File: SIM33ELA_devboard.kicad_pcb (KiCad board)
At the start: 4 copper layers, 82.3 x 24.9 mm, 26 parts, among them J2 Conn_01x13_Pin, U2 SIM33ELA

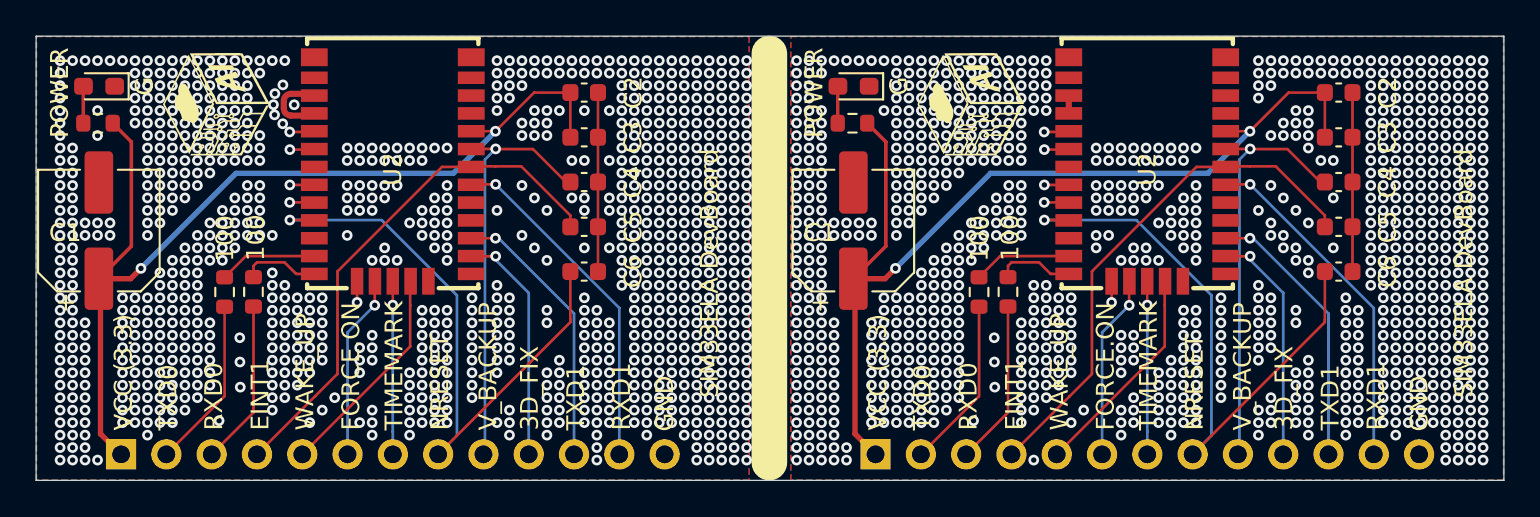
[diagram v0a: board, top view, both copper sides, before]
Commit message: cambios finales
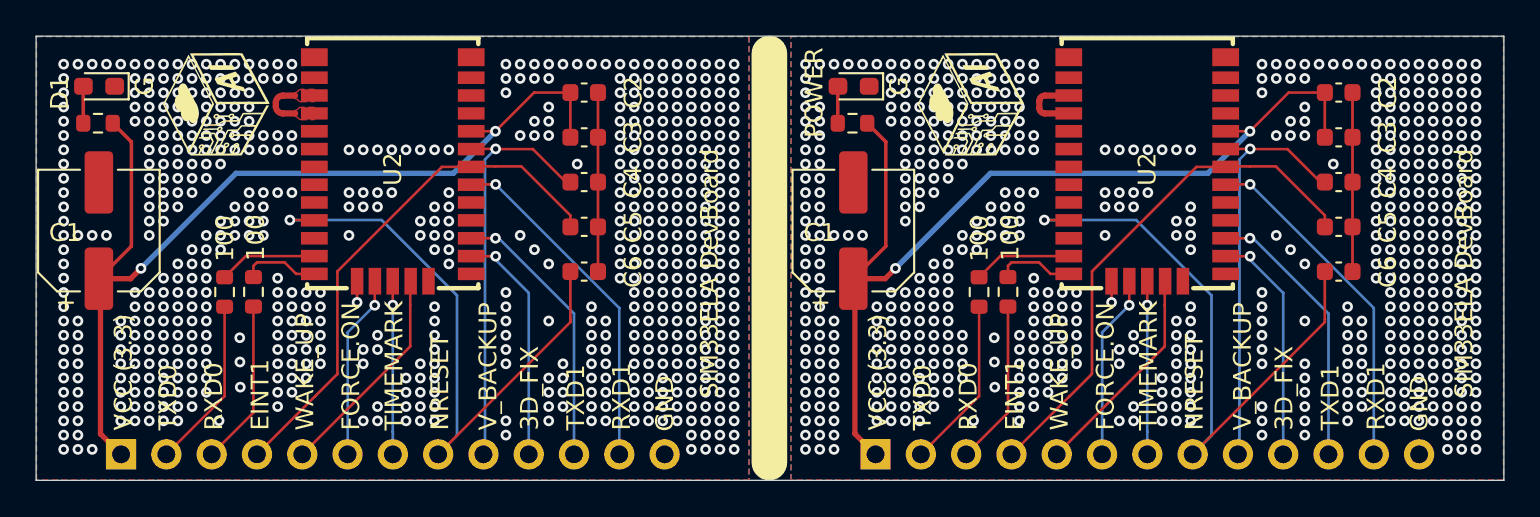
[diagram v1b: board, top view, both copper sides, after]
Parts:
- R3: value 2.7k -> 4.7k
- renumbered POWER to D1
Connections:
- U2 pad 16: Net-(U2-ANT) -> /RF_SIGNAL1
- U2 pad 17: Net-(U2-ANT) -> /RF_SIGNAL1
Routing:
- net GND: track 33.3 -> 22.5 mm, vias 1886 -> 1201
- net /RF_SIGNAL1: track 0.00 -> 4.14 mm
- net Net-(U2-ANT): track 6.56 -> 4.02 mm
- added copper zone on F.Cu, net /RF_SIGNAL1

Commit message: diseño final
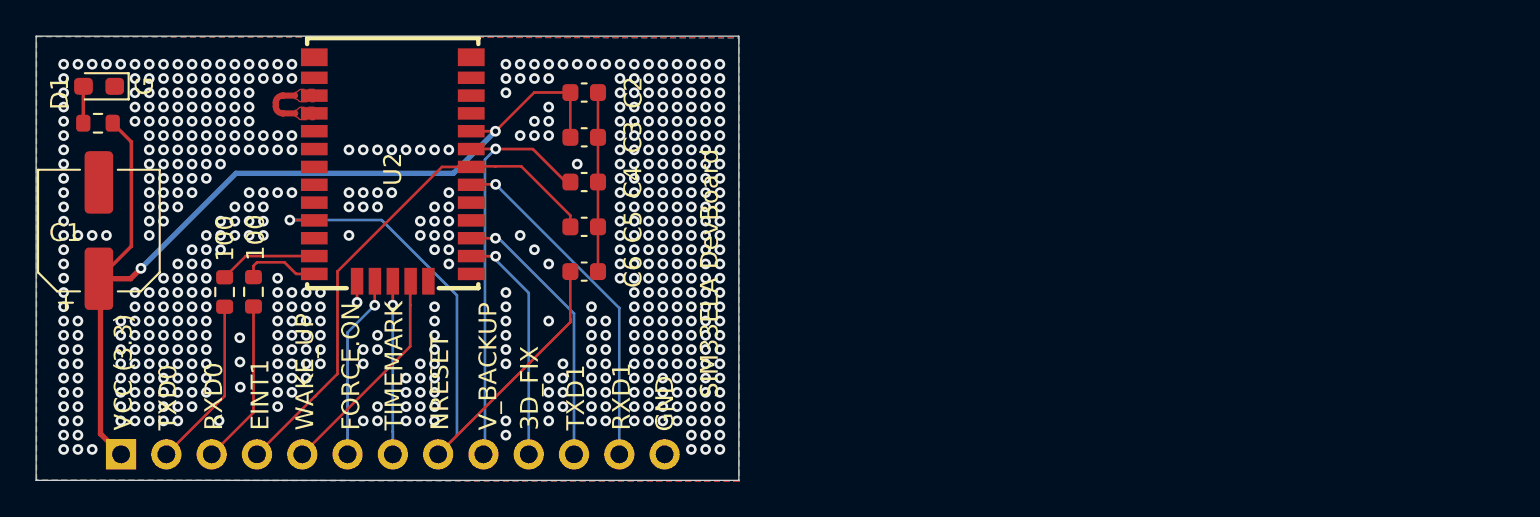
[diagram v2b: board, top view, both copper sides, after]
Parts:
- removed the C1 at (170.6, 91.8)
- removed the C2 at (197.8, 84.0)
- removed the C3 at (197.8, 86.5)
- removed the C4 at (197.8, 89.0)
- removed the C5 at (197.8, 91.5)
- removed the C6 at (197.8, 94.1)
- removed G*** (x2): LOGO, Images:LOGOv3.4
- removed the J2 at (171.8, 104.3)
- removed POWER: LED_Small, LED_SMD:LED_0603_1608Metric_Pad1.05x0.95mm_HandSolder
- removed the R1 at (179.3, 95.2)
- removed the R2 at (177.7, 95.2)
- removed the R3 at (170.6, 85.7)
- removed the U2 at (187.1, 88.3)
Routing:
- net /VCC: track 109.7 -> 54.9 mm, vias 4 -> 2
- net /NRESET: track 70.3 -> 35.2 mm, vias 2 -> 1
- net /EINT1: track 58.8 -> 29.4 mm
- net /V_BAKCUP: track 47.5 -> 23.7 mm, vias 2 -> 1
- net /RXD1: track 38.7 -> 19.4 mm, vias 2 -> 1
- net /TXD1: track 30.8 -> 15.4 mm, vias 2 -> 1
- net /3D-FIX: track 26.5 -> 13.2 mm, vias 2 -> 1
- net /WAKE_UP: track 24.5 -> 12.2 mm
- net GND: track 22.5 -> 11.2 mm, vias 1201 -> 581
- net /FORCE_ON: track 20.7 -> 10.4 mm, vias 2 -> 1
- net /TIMEMARK: track 19.5 -> 9.73 mm, vias 2 -> 1
- net /TXD0: track 19.3 -> 9.63 mm
- net /RXD0: track 18.5 -> 9.26 mm
- net Net-(U2-TXD0): track 11.0 -> 5.52 mm
- net Net-(U2-RXD0): track 8.78 -> 4.39 mm
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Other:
- board size 82.3 x 24.9 mm -> 39.4 x 24.9 mm
- board text removed: "recto"

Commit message: aaa
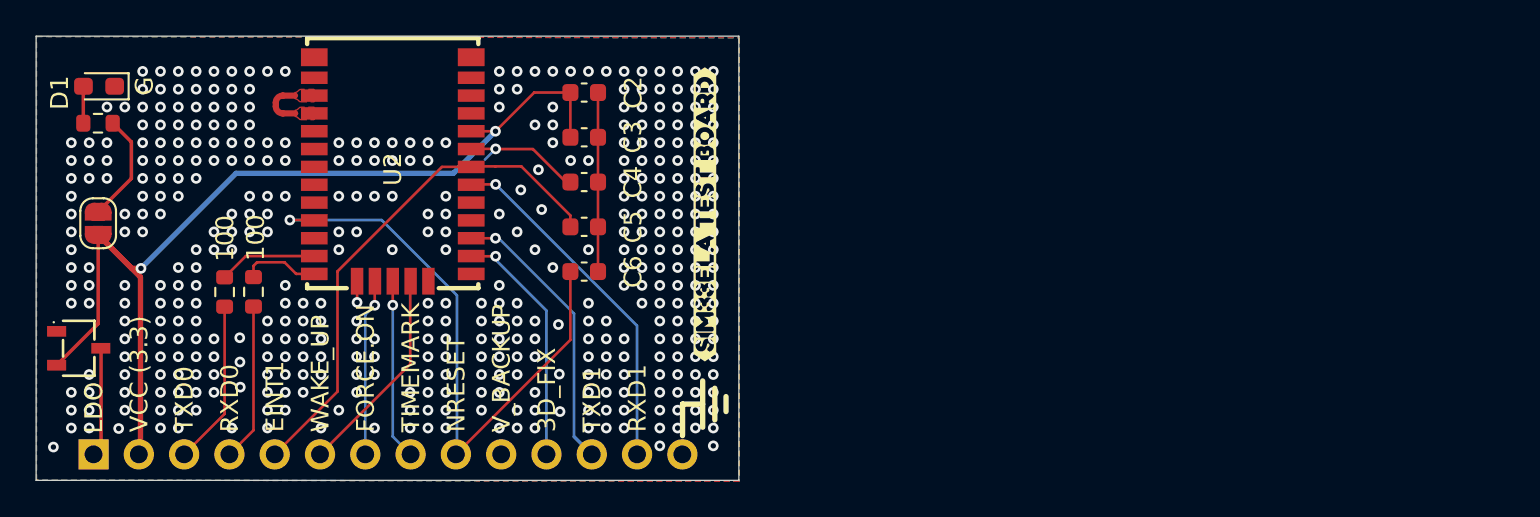
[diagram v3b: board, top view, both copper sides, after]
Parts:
- removed C1: 470uF, Capacitor_SMD:CP_Elec_6.3x7.7
- removed J2: Conn_01x13_Pin, Connector_PinHeader_2.54mm:PinHeader_1x13_P2.54mm_Vertical
- added J1: Conn_01x14_Pin, Connector_PinHeader_2.54mm:PinHeader_1x14_P2.54mm_Vertical, B.Cu at (128.0, 104.3)
- added JP1: SolderJumper_2_Open, Jumper:SolderJumper-2_P1.3mm_Open_RoundedPad1.0x1.5mm, F.Cu at (128.2, 91.3)
- added U1: XC6206P332MR, EasyEDA:SOT-23-3_L2.9-W1.6-P1.90-LS2.8-BR, F.Cu at (127.2, 98.4)
- added kibuzzard-6A1C62F4: G***, kibuzzard-6A1C62F4, F.Cu at (162.3, 90.8)
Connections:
- R3 pad 2: /VCC -> Net-(JP1-A)
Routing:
- net /V_BAKCUP: track 23.7 -> 7.17 mm
- net Net-(JP1-A): track 0.00 -> 6.16 mm
- net /LDO: track 0.00 -> 6.13 mm
- net /VCC: track 54.9 -> 56.9 mm
- net /NRESET: track 35.2 -> 34.3 mm
- net GND: vias 581 -> 420
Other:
- board text added: "LDO"
- board text removed: "GND"
- board text removed: "SIM33ELA DevBoard"
